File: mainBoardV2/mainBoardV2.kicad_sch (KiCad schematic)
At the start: 34 parts, among them J1 USB4125-GF-A_REVA2, SW1 SW_SPST, U1 ESP32-CAM, U2 ESP32-DEVKITC-32E, U3 MCP73871-2AAI_ML, U4 MPU6050_Module, U5 TPS61090RSARG4

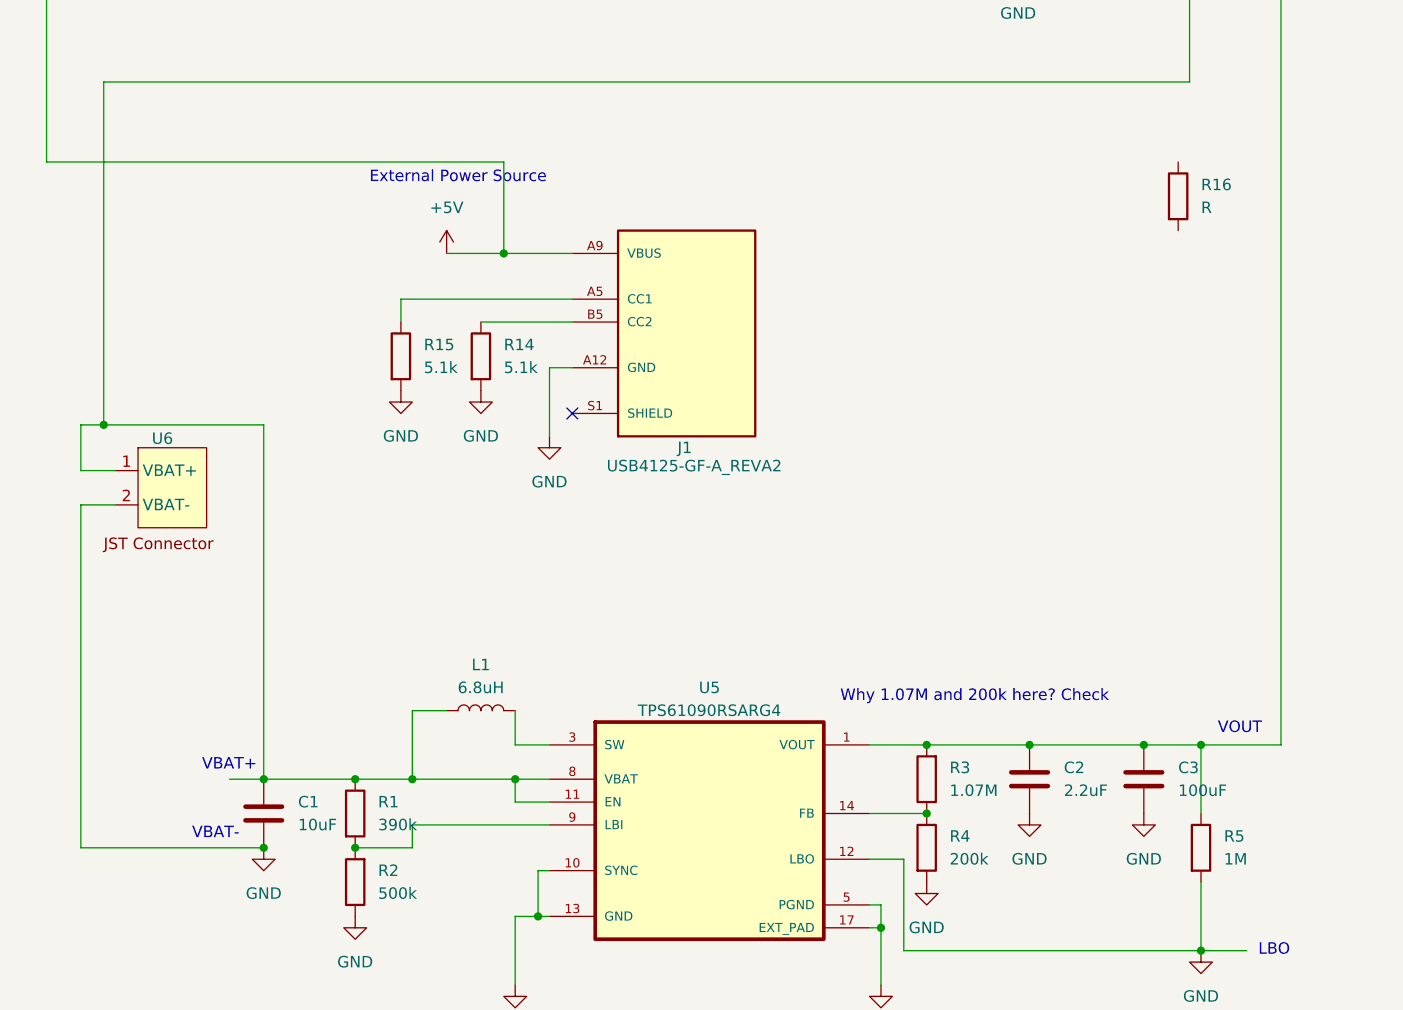
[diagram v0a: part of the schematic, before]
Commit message: 2.28.26.C3
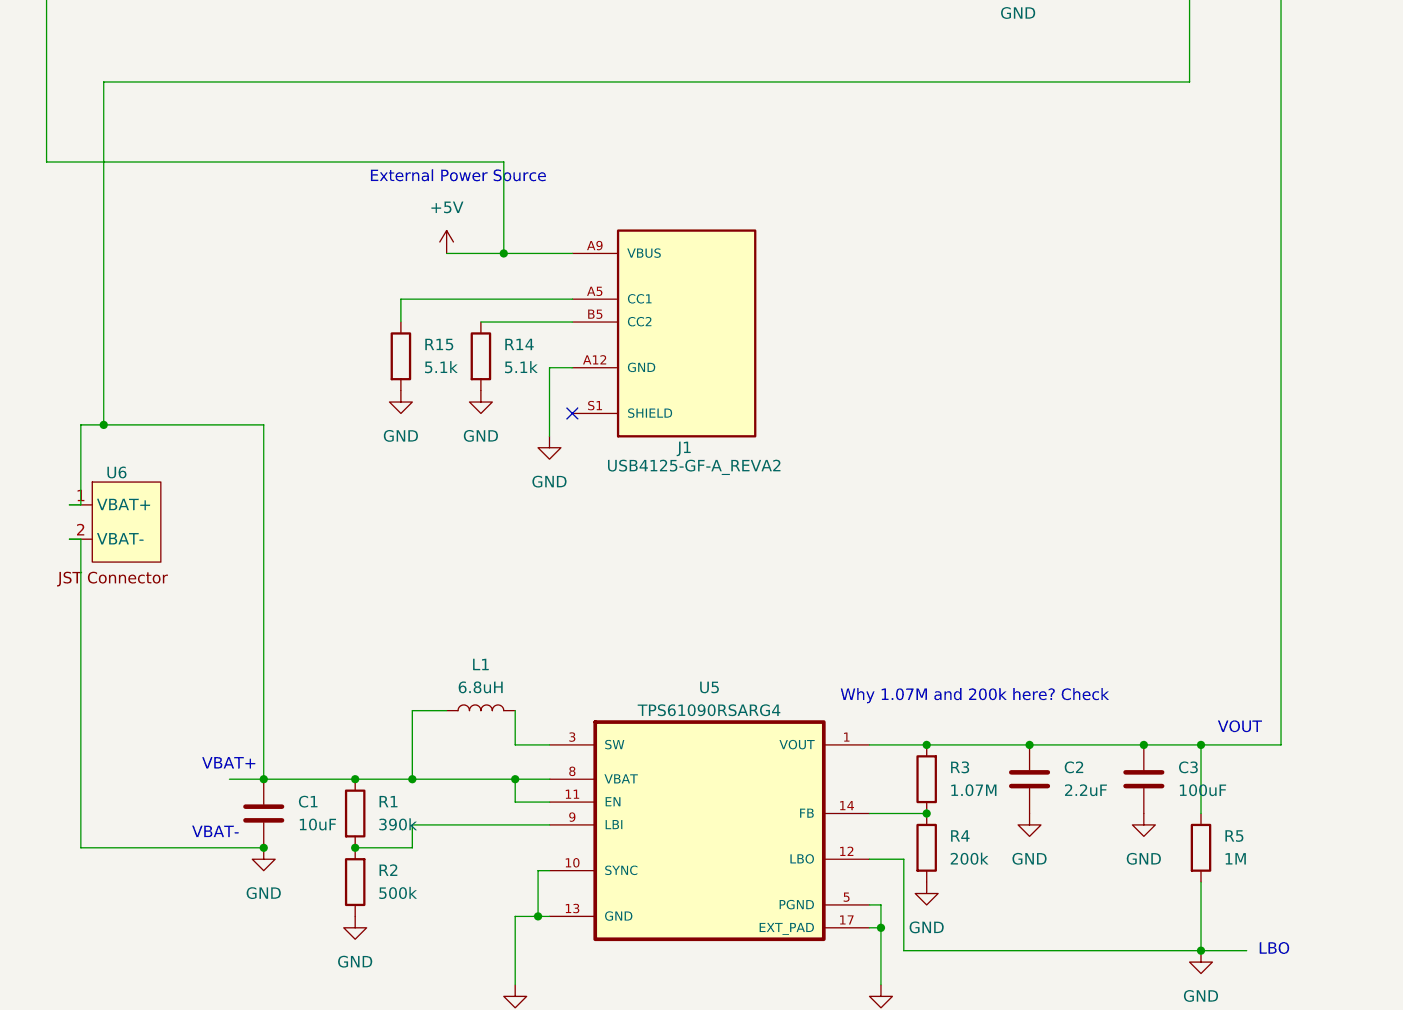
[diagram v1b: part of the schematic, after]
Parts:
- removed R16: R, symbol Device:R
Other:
- moved on the sheet: U6
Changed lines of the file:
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@@
 	(wire
 		(pts
-			(xy 25.4 125.73) (xy 21.59 125.73)
+			(xy 20.32 129.54) (xy 21.59 129.54)
 		)
 		(stroke
@@
 	(wire
 		(pts
-			(xy 21.59 125.73) (xy 21.59 120.65)
+			(xy 21.59 129.54) (xy 21.59 120.65)
 		)
 		(stroke
@@
 	(wire
 		(pts
-			(xy 25.4 129.54) (xy 21.59 129.54)
+			(xy 20.32 133.35) (xy 21.59 133.35)
 		)
 		(stroke
@@
 	(wire
 		(pts
-			(xy 21.59 129.54) (xy 21.59 167.64)
+			(xy 21.59 133.35) (xy 21.59 167.64)
 		)
 		(stroke
@@
 	(symbol
 		(lib_id "Device:R")
-		(at 143.51 95.25 0)
-		(unit 1)
-		(exclude_from_sim no)
-		(in_bom yes)
-		(on_board yes)
-		(dnp no)
-		(fields_autoplaced yes)
-		(property "Reference" "R16"
-			(at 146.05 93.9799 0)
-			(effects
-				(font
-					(size 1.27 1.27)
-				)
-				(justify left)
-			)
-		)
-		(property "Value" "R"
-			(at 146.05 96.5199 0)
-			(effects
-				(font
-					(size 1.27 1.27)
-				)
-				(justify left)
-			)
-		)
-		(property "Footprint" ""
-			(at 141.732 95.25 90)
-			(effects
-				(font
-					(size 1.27 1.27)
-				)
-				(hide yes)
-			)
-		)
-		(property "Datasheet" "~"
-			(at 143.51 95.25 0)
-			(effects
-				(font
-					(size 1.27 1.27)
-				)
-				(hide yes)
-			)
-		)
-		(property "Description" "Resistor"
-			(at 143.51 95.25 0)
-			(effects
-				(font
-					(size 1.27 1.27)
-				)
-				(hide yes)
-			)
-		)
-		(pin "1"
-		)
-		(pin "2"
-		)
-		(instances
-			(project ""
-				(path "/7ab8875a-49c9-4be9-9bdd-57c13261595f"
-					(reference "R16")
-					(unit 1)
-				)
-			)
-		)
-	)
-	(symbol
-		(lib_id "Device:R")
 		(at 66.04 113.03 0)
 		(unit 1)
@@
 	(symbol
 		(lib_id "Connector:JST_2pin_2mm")
-		(at 29.21 121.92 0)
+		(at 24.13 125.73 0)
 		(unit 1)
 		(exclude_from_sim no)
@@
 		(dnp no)
 		(property "Reference" "U6"
-			(at 29.464 122.174 0)
+			(at 24.384 125.984 0)
 			(effects
 				(font
@@
 		)
 		(property "Value" "~"
-			(at 38.1 130.3047 0)
+			(at 33.02 134.1147 0)
 			(effects
 				(font
@@
 		)
 		(property "Footprint" "Connector_JST:JST_PH_S2B-PH-K_1x02_P2.00mm_Horizontal"
-			(at 29.21 121.92 0)
+			(at 24.13 125.73 0)
 			(effects
 				(font
@@
 		)
 		(property "Datasheet" ""
-			(at 29.21 121.92 0)
+			(at 24.13 125.73 0)
 			(effects
 				(font
@@
 		)
 		(property "Description" ""
-			(at 29.21 121.92 0)
+			(at 24.13 125.73 0)
 			(effects
 				(font
